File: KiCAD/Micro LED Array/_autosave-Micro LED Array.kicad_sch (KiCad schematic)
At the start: 15 parts, among them J1 Conn_02x07_1mm

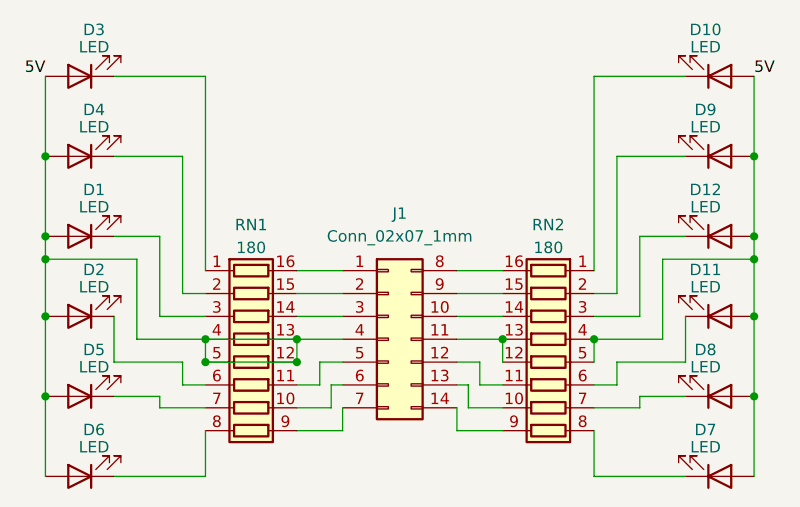
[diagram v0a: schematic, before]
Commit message: Working draft
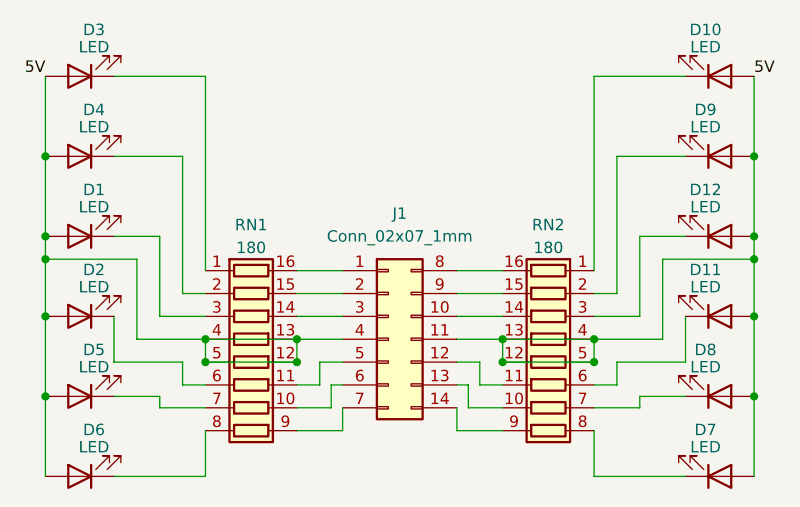
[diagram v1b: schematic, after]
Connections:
- net 5V: now also J1.11 (Pin_11), RN2.12 (R5.2), RN2.13 (R4.2)
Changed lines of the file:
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@@
   (junction (at 114.3 91.44) (diameter 0) (color 0 0 0 0)
+  )
+  (junction (at 137.16 91.44) (diameter 0) (color 0 0 0 0)
   )
   (junction (at 104.14 88.9) (diameter 0) (color 0 0 0 0)
   )
   (junction (at 165.1 86.36) (diameter 0) (color 0 0 0 0)
+  )
+  (junction (at 147.32 91.44) (diameter 0) (color 0 0 0 0)
   )
   (junction (at 86.36 68.58) (diameter 0) (color 0 0 0 0)
@@
     (stroke (width 0) (type default))
   )
+  (wire (pts (xy 137.16 88.9) (xy 147.32 88.9))
+    (stroke (width 0) (type default))
+  )
   (wire (pts (xy 101.6 93.98) (xy 104.14 93.98))
     (stroke (width 0) (type default))
@@
     (stroke (width 0) (type default))
   )
+  (wire (pts (xy 137.16 91.44) (xy 147.32 91.44))
+    (stroke (width 0) (type default))
+  )
